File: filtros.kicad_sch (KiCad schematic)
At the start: 24 parts, among them U1 ${SIM.PARAMS}, U2 ${SIM.PARAMS}, U3 ${SIM.PARAMS}, U4 ${SIM.PARAMS}

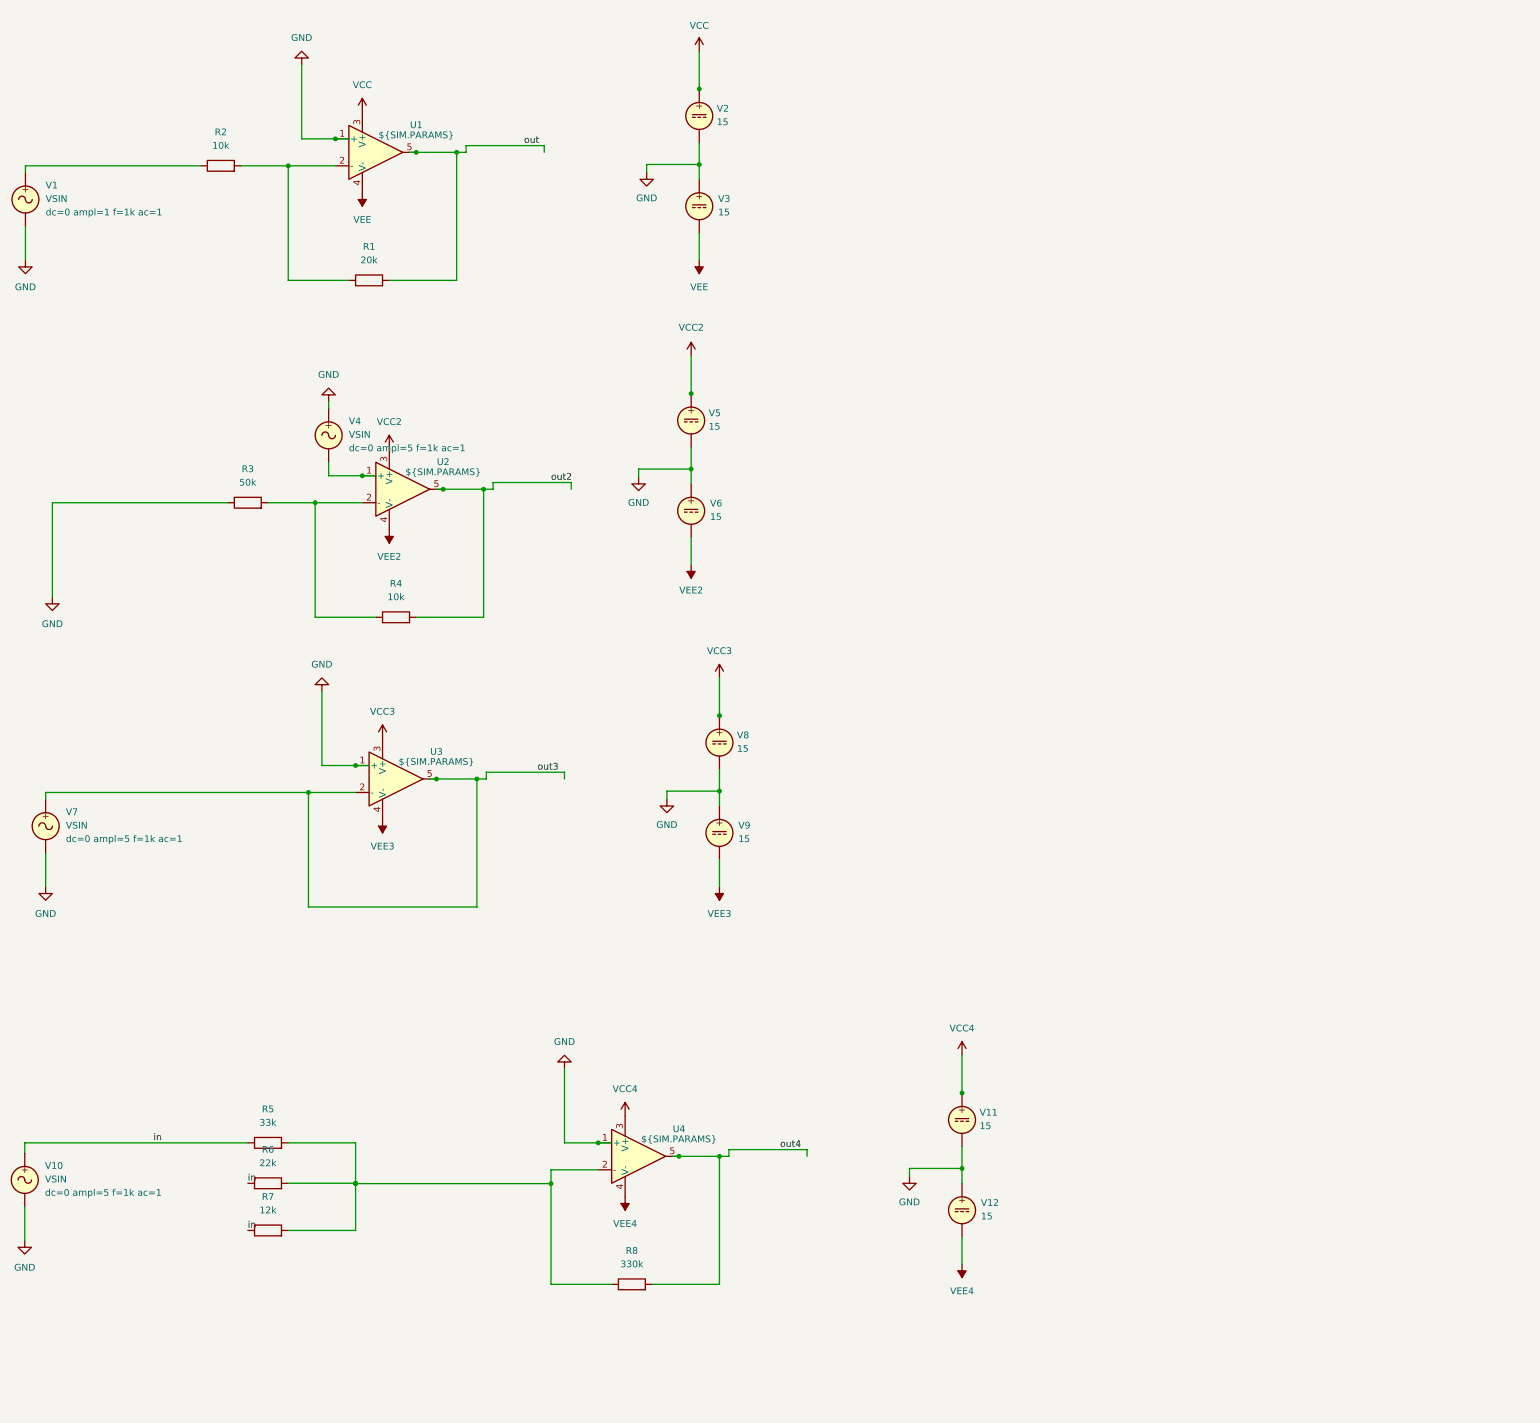
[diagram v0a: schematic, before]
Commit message: updates
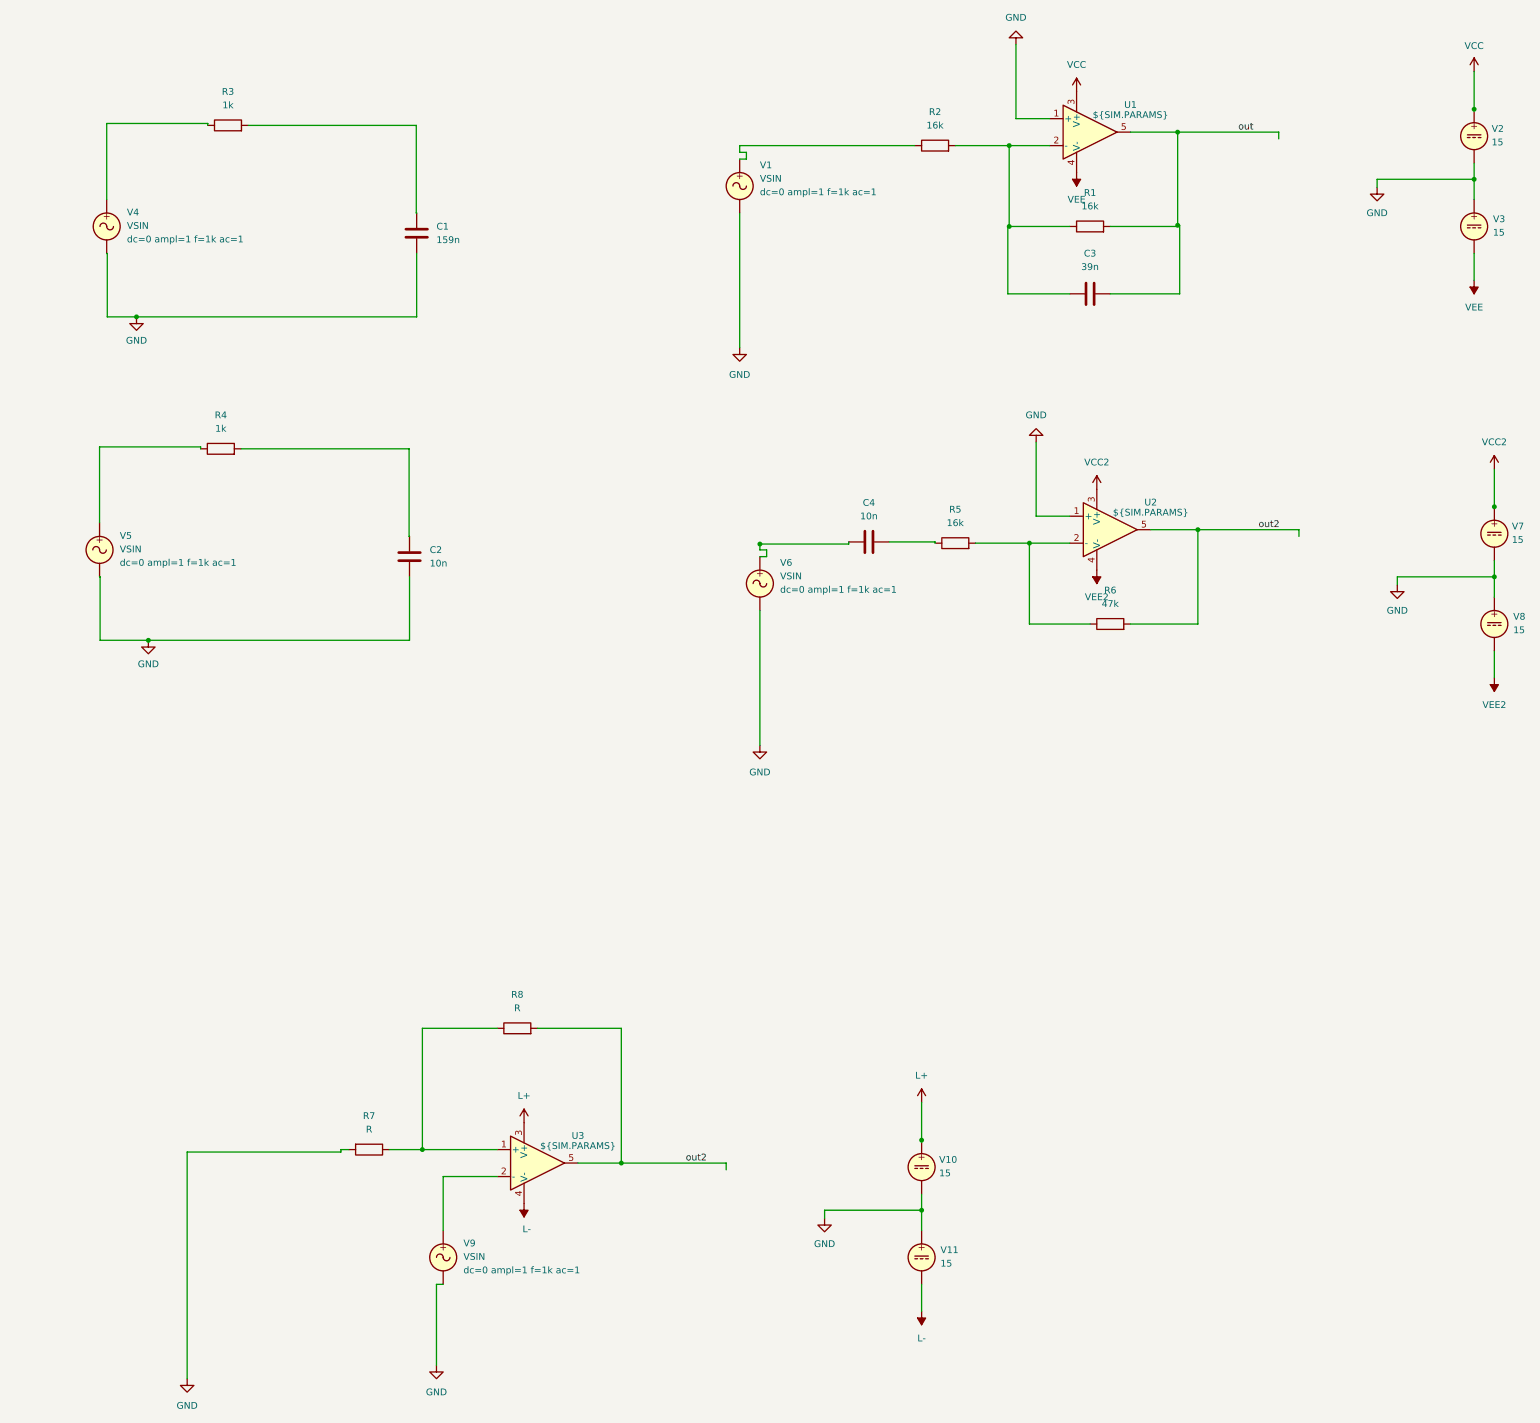
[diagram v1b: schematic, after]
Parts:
- removed U4: ${SIM.PARAMS}, symbol Simulation_SPICE:OPAMP
- removed V10, V7: VSIN, symbol Simulation_SPICE:VSIN
- removed V12, V5, V6, V9: 15, symbol Simulation_SPICE:VDC
- added C1: 159n, symbol Device:C
- added C2, C4: 10n, symbol Device:C
- added C3: 39n, symbol Device:C
- added V10, V7: 15, symbol Simulation_SPICE:VDC
- added V5, V6, V9: VSIN, symbol Simulation_SPICE:VSIN
- R1: value 20k -> 16k
- R2: value 10k -> 16k
- R3: value 50k -> 1k
- R4: value 10k -> 1k
- R5: value 33k -> 16k
- R6: value 22k -> 47k
- R7: value 12k -> R
- R8: value 330k -> R
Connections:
- net VCC4 is gone; now on net GND: V11.1
- net out4 is gone; now on net out2: R8.2
- net GND: now also R7.2, U2.1 (+), V4.2, V8.1, C1.2, C2.2, V10.2, V5.2, V6.2, V7.2, V9.2; no longer R3.1, U3.1 (+), V11.2, V4.1, V8.2
- net VCC2: now also V7.1
- net VEE2: now also V8.2
- net out: now also C3.2
- net out2: now also R6.2, U3.5; no longer R4.2
- net at R1.1, R2.2, U1.2 (-): now also C3.1
- net VCC3 renamed L+
- net L+: now also V10.1; no longer V8.1
- net VEE3 renamed L-
- net L-: now also V11.2
- removed net in: R5.1, R6.1, R7.1
- net out3: no longer names the net of U3.2 (-)
- net out3: now also V9.1; no longer U3.5
- new net: C1.1, R3.2
- new net: R7.1, R8.1, U3.1 (+)
- new net: R5.2, R6.1, U2.2 (-)
- new net: C4.1, V6.1
- new net: R4.1, V5.1
- new net: C2.1, R4.2
- new net: C4.2, R5.1
- new net: R3.1, V4.1
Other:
- moved on the sheet: R1, R2, U1, V1, V2, V3
